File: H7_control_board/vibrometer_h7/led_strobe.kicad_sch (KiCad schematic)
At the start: 47 parts, among them Q1001 NMOS, Q1002 NMOS, Q1003 NMOS

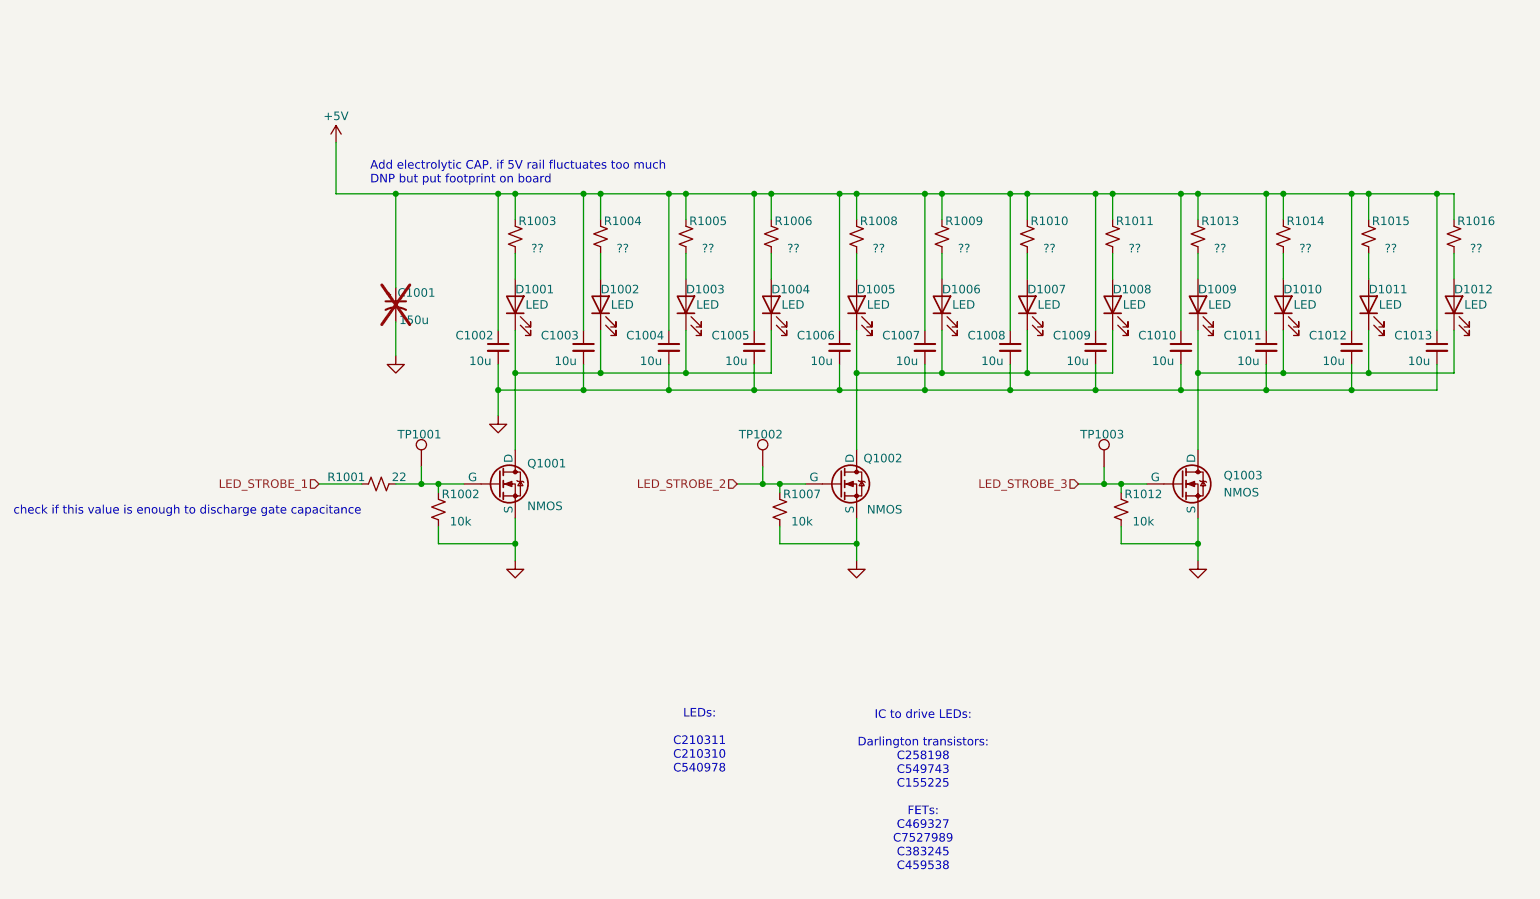
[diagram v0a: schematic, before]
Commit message: lots of routing progress!!
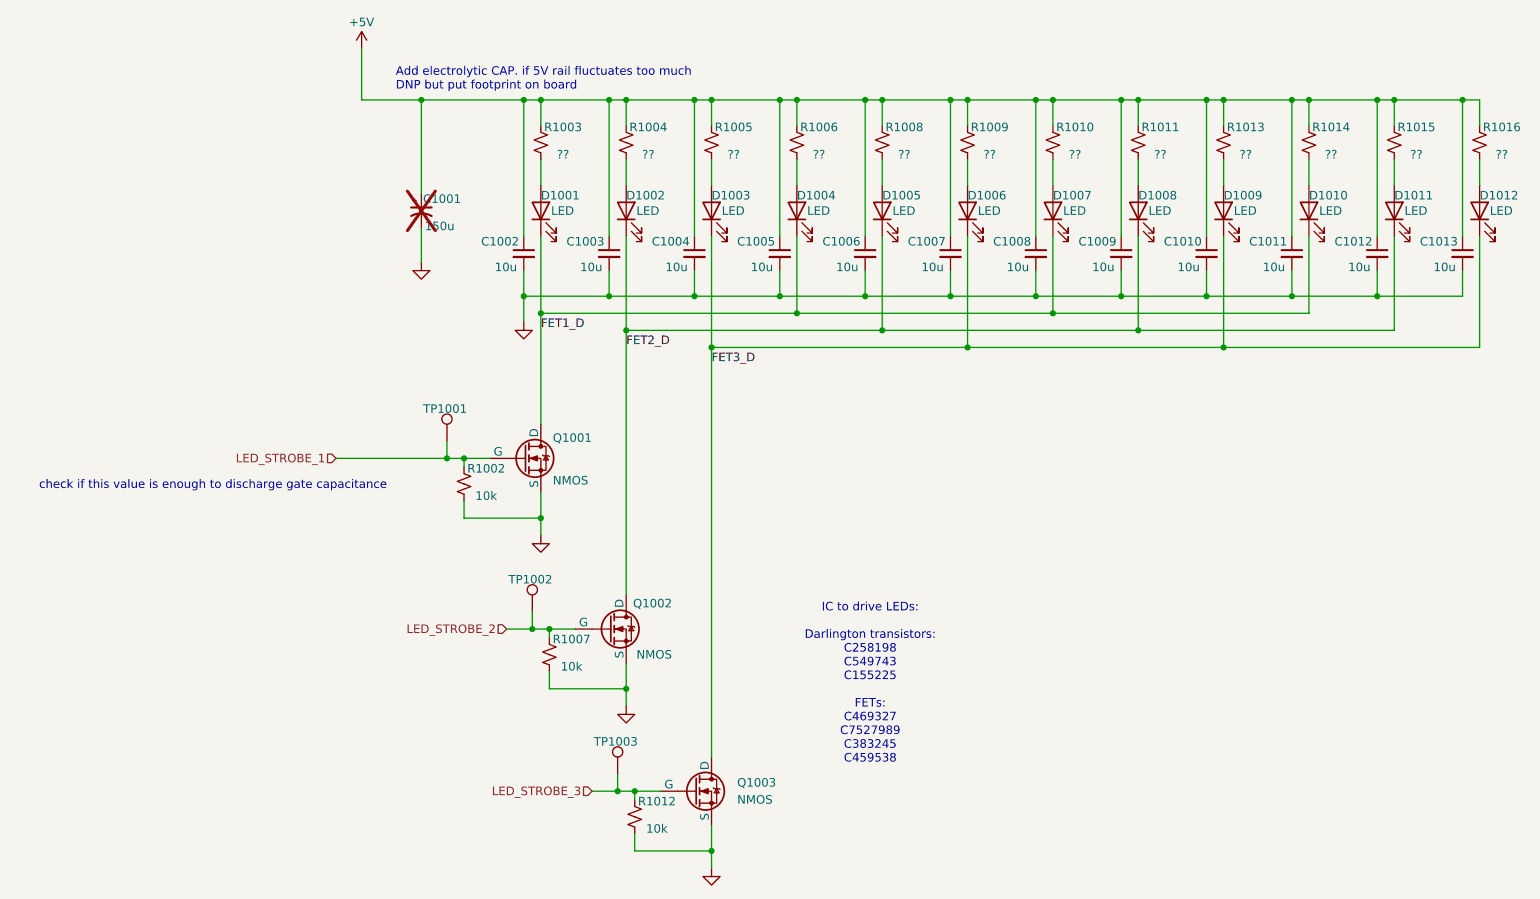
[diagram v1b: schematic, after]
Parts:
- removed R1001: 22, Resistor_SMD:R_0402_1005Metric, symbol Device:R_Small_US
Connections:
- net LED_STROBE_1: now also Q1001.2 (G), R1002.2, TP1001.1
- net FET2_D: now reaches D1005.1 (K), D1008.1 (K), Q1002.1 (D)
- net FET2_D: now also D1002.1 (K), D1011.1 (K); no longer D1006.1 (K), D1007.1 (K)
- net FET1_D: now reaches D1001.1 (K), D1004.1 (K), Q1001.1 (D)
- net FET1_D: now also D1007.1 (K), D1010.1 (K); no longer D1002.1 (K), D1003.1 (K)
- net FET3_D: now reaches D1009.1 (K), D1012.1 (K), Q1003.1 (D)
- net FET3_D: now also D1003.1 (K), D1006.1 (K); no longer D1010.1 (K), D1011.1 (K)
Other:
- note removed: "LEDs: C210311 C210310 C540978"
- moved on the sheet: C1001, C1002, C1003, C1004, C1005, C1006, C1007, C1008, C1009, C1010, C1011, C1012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
